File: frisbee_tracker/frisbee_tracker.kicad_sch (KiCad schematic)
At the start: 63 parts, among them IC1 NRF54L05-QFAA-R7, J1 UJC-H-G-SMT-2-P6-TR, J2 FTSH-105-01-L-DV-K, U1 AP2210N-3.3TRG1, U2 BQ24072RGTT, U3 BMI323, U4 BSS138, U5 BSS138, U6 BSS138, U7 BSS138, Y1 32 MHz, Y2 32.768 kHz

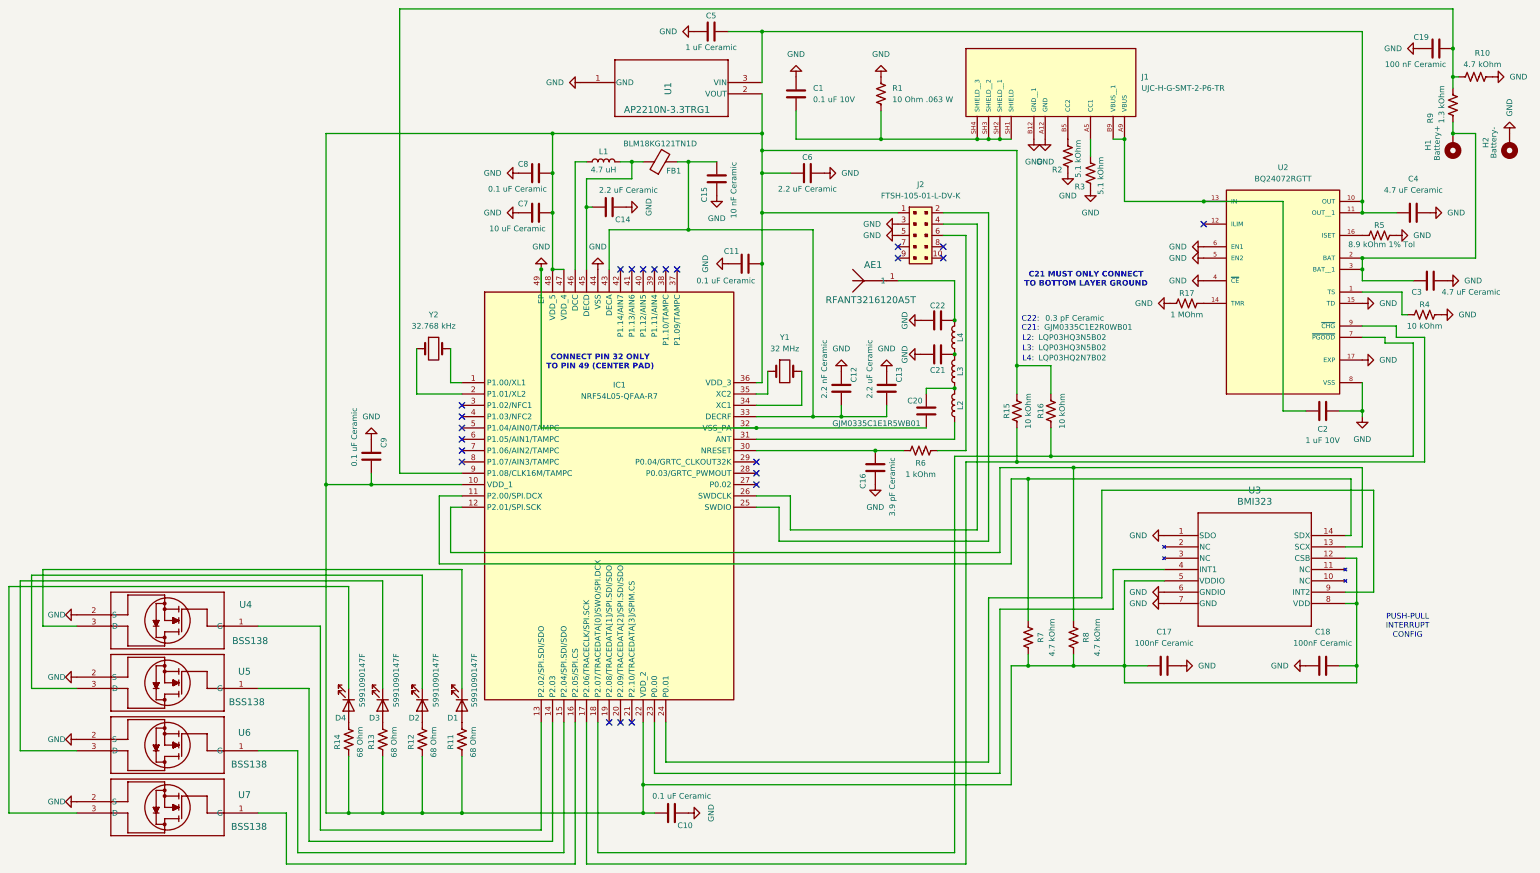
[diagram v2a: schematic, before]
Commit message: PCB design 90% complete
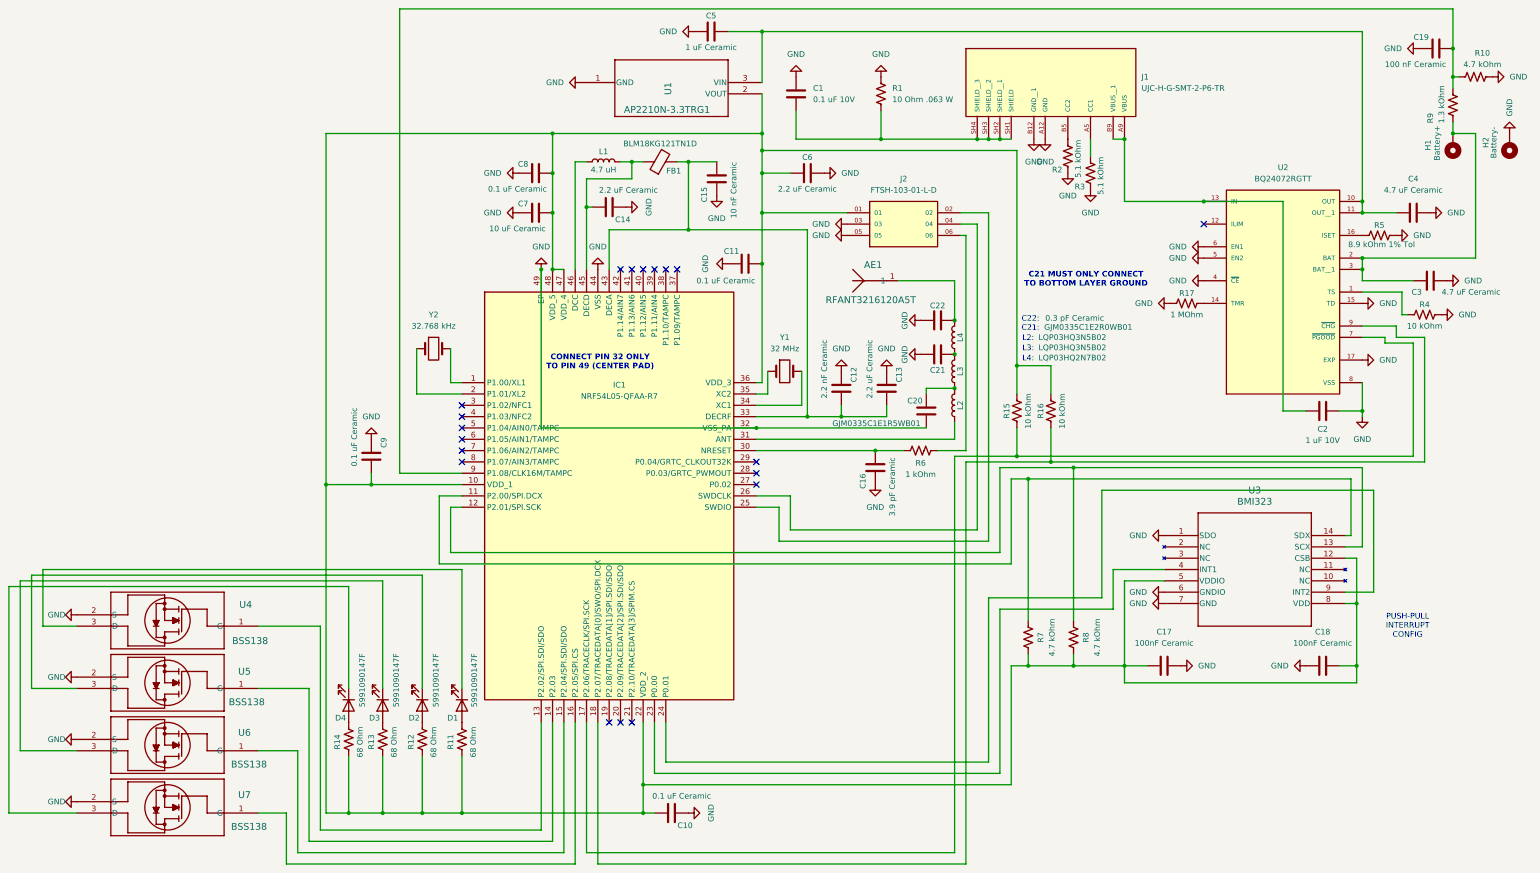
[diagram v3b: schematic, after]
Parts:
- removed J2: FTSH-105-01-L-DV-K, footprints:FTSH-105-01-L-DV-K, symbol dk_Rectangular-Connectors-Headers-Male-Pins:FTSH-105-01-L-DV-K
- added J2: FTSH-103-01-L-D, footprints:FTSH-103-01-L-D, symbol FTSH-103-01-L-D:FTSH-103-01-L-D
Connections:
- net GND: now also J2.03, J2.05
- net at C10.2, C11.2, C17.1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: now also J2.01
- net at IC1.18 (P2.07/TRACEDATA[0]/SWO/SPI.DCX), R16.1: now also U2.9 (~{CHG}); no longer U2.7 (~{PGOOD})
- net at IC1.17 (P2.06/TRACECLK/SPI.SCK), R15.1: now also U2.7 (~{PGOOD}); no longer U2.9 (~{CHG})
- net at R6.2: now also J2.06
- net at IC1.25 (SWDIO): now also J2.02
- net at IC1.26 (SWDCLK): now also J2.04
- no-connect marks 23 -> 19

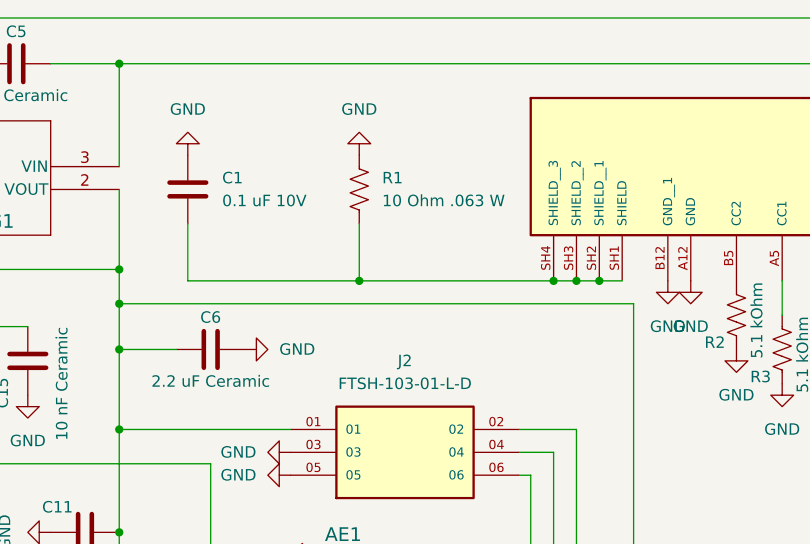
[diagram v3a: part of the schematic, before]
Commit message: Rough draft of PCB completed
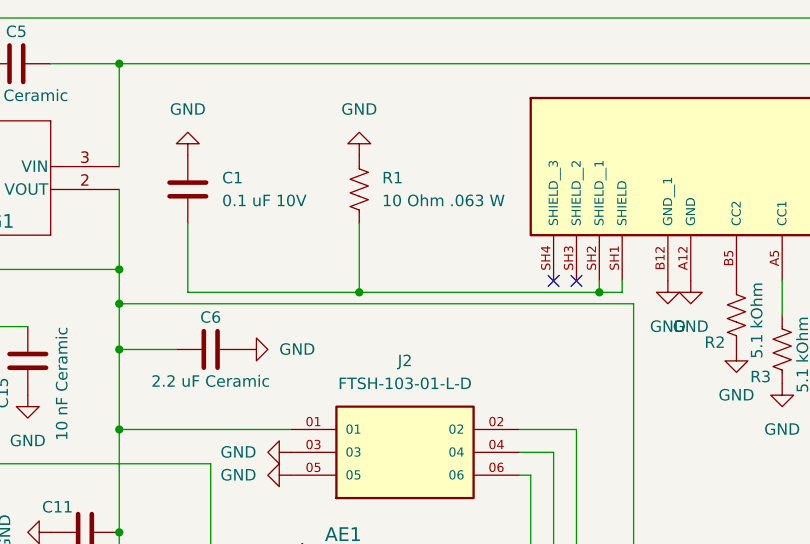
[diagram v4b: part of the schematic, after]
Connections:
- net at C1.2, J1.SH1 (SHIELD), J1.SH2 (SHIELD__1)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: no longer J1.SH3 (SHIELD__2), J1.SH4 (SHIELD__3)
- no-connect marks 19 -> 21
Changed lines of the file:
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@@
+	)
+	(junction
+		(at 165.1 43.18)
+		(diameter 0)
+		(color 0 0 0 0)
 	)
 	(junction
@@
 	)
 	(junction
-		(at 162.56 41.91)
-		(diameter 0)
-		(color 0 0 0 0)
-	)
-	(junction
 		(at 111.76 49.53)
 		(diameter 0)
@@
 	)
 	(junction
+		(at 138.43 43.18)
+		(diameter 0)
+		(color 0 0 0 0)
+	)
+	(junction
 		(at 111.76 40.64)
 		(diameter 0)
@@
 	)
 	(junction
-		(at 138.43 41.91)
-		(diameter 0)
-		(color 0 0 0 0)
-	)
-	(junction
 		(at 181.61 160.02)
 		(diameter 0)
@@
 	)
 	(junction
-		(at 160.02 41.91)
-		(diameter 0)
-		(color 0 0 0 0)
-	)
-	(junction
 		(at 44.45 193.04)
 		(diameter 0)
@@
 	(junction
 		(at 266.7 27.94)
-		(diameter 0)
-		(color 0 0 0 0)
-	)
-	(junction
-		(at 165.1 41.91)
 		(diameter 0)
 		(color 0 0 0 0)
@@
 	)
 	(no_connect
+		(at 160.02 41.91)
+	)
+	(no_connect
 		(at 44.45 109.22)
 	)
@@
 	)
 	(no_connect
+		(at 162.56 41.91)
+	)
+	(no_connect
 		(at 44.45 111.76)
 	)
@@
 	(wire
 		(pts
+			(xy 167.64 43.18) (xy 167.64 41.91)
+		)
+		(stroke
+			(width 0)
+			(type default)
+		)
+	)
+	(wire
+		(pts
 			(xy 67.31 172.72) (xy 67.31 201.93)
 		)
@@
 	(wire
 		(pts
-			(xy 165.1 41.91) (xy 167.64 41.91)
+			(xy 165.1 43.18) (xy 167.64 43.18)
 		)
 		(stroke
@@
 	(wire
 		(pts
-			(xy 119.38 35.56) (xy 119.38 41.91)
+			(xy 119.38 35.56) (xy 119.38 43.18)
 		)
 		(stroke
@@
 	(wire
 		(pts
-			(xy 119.38 41.91) (xy 138.43 41.91)
+			(xy 119.38 43.18) (xy 138.43 43.18)
 		)
 		(stroke
@@
 	(wire
 		(pts
-			(xy 160.02 41.91) (xy 162.56 41.91)
-		)
-		(stroke
-			(width 0)
-			(type default)
-		)
-	)
-	(wire
-		(pts
 			(xy 246.38 133.35) (xy 242.57 133.35)
 		)
@@
 	(wire
 		(pts
+			(xy 165.1 41.91) (xy 165.1 43.18)
+		)
+		(stroke
+			(width 0)
+			(type default)
+		)
+	)
+	(wire
+		(pts
 			(xy 120.65 101.6) (xy 120.65 93.98)
 		)
@@
 	(wire
 		(pts
-			(xy 138.43 41.91) (xy 138.43 35.56)
-		)
-		(stroke
-			(width 0)
-			(type default)
-		)
-	)
-	(wire
-		(pts
 			(xy 246.38 17.78) (xy 111.76 17.78)
 		)
@@
 	(wire
 		(pts
-			(xy 162.56 41.91) (xy 165.1 41.91)
-		)
-		(stroke
-			(width 0)
-			(type default)
-		)
-	)
-	(wire
-		(pts
 			(xy 246.38 115.57) (xy 246.38 133.35)
 		)
@@
 	(wire
 		(pts
+			(xy 165.1 43.18) (xy 138.43 43.18)
+		)
+		(stroke
+			(width 0)
+			(type default)
+		)
+	)
+	(wire
+		(pts
 			(xy 69.85 204.47) (xy 69.85 172.72)
 		)
@@
 	(wire
 		(pts
+			(xy 138.43 35.56) (xy 138.43 43.18)
+		)
+		(stroke
+			(width 0)
+			(type default)
+		)
+	)
+	(wire
+		(pts
 			(xy 111.76 44.45) (xy 111.76 49.53)
 		)
@@
 		)
 		(stroke
-			(width 0)
-			(type default)
-		)
-	)
-	(wire
-		(pts
-			(xy 138.43 41.91) (xy 160.02 41.91)
-		)
-		(stroke
